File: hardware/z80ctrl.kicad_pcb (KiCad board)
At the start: 2 copper layers, 99.8 x 49.9 mm, 28 parts, among them J1 BUS, J2 BUSEXT, J4 IOADDR, J5 SERIAL1, J6 SERIAL2, J7 SD, SW1 RESET, SW2 HALT, U1 74HCT139, U2 ATMEGA1284P-PU, U3 74HCT74, U4 MCP23S17, Y1 20MHz

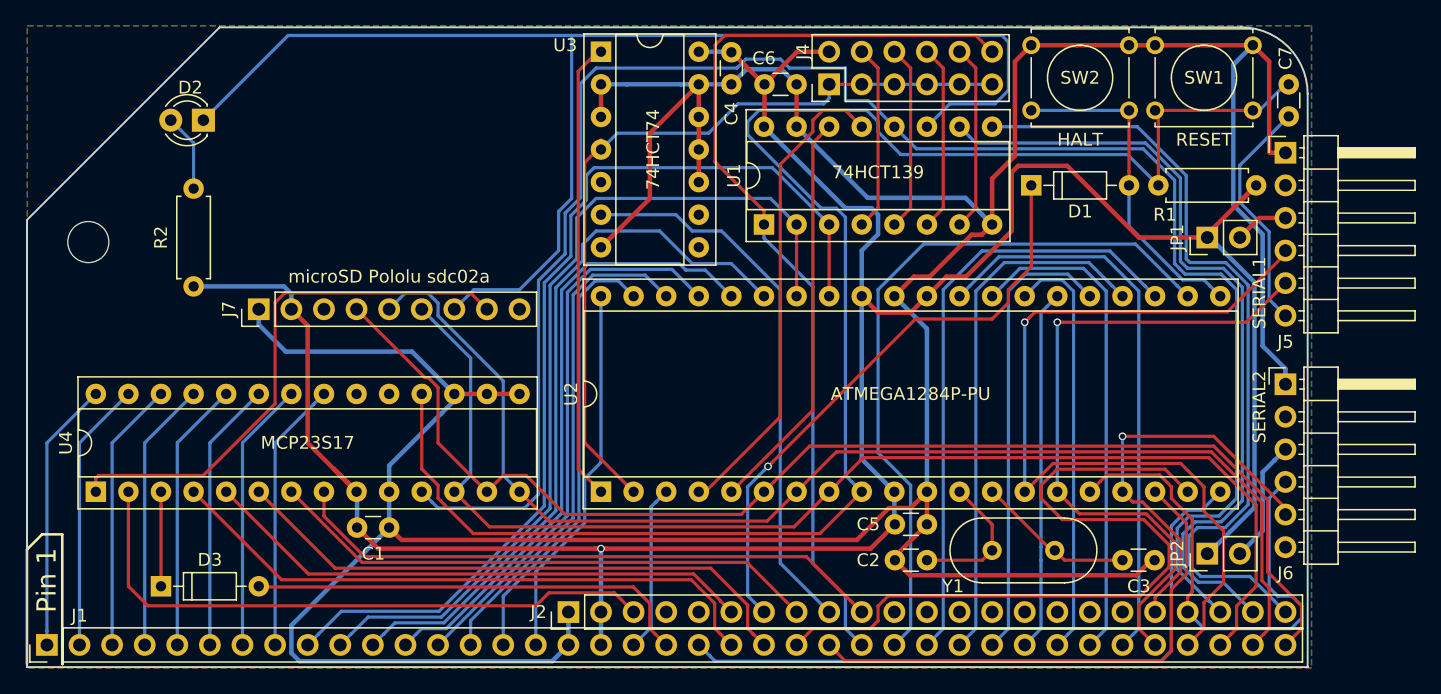
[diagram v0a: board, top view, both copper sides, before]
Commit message: OCD tweaks
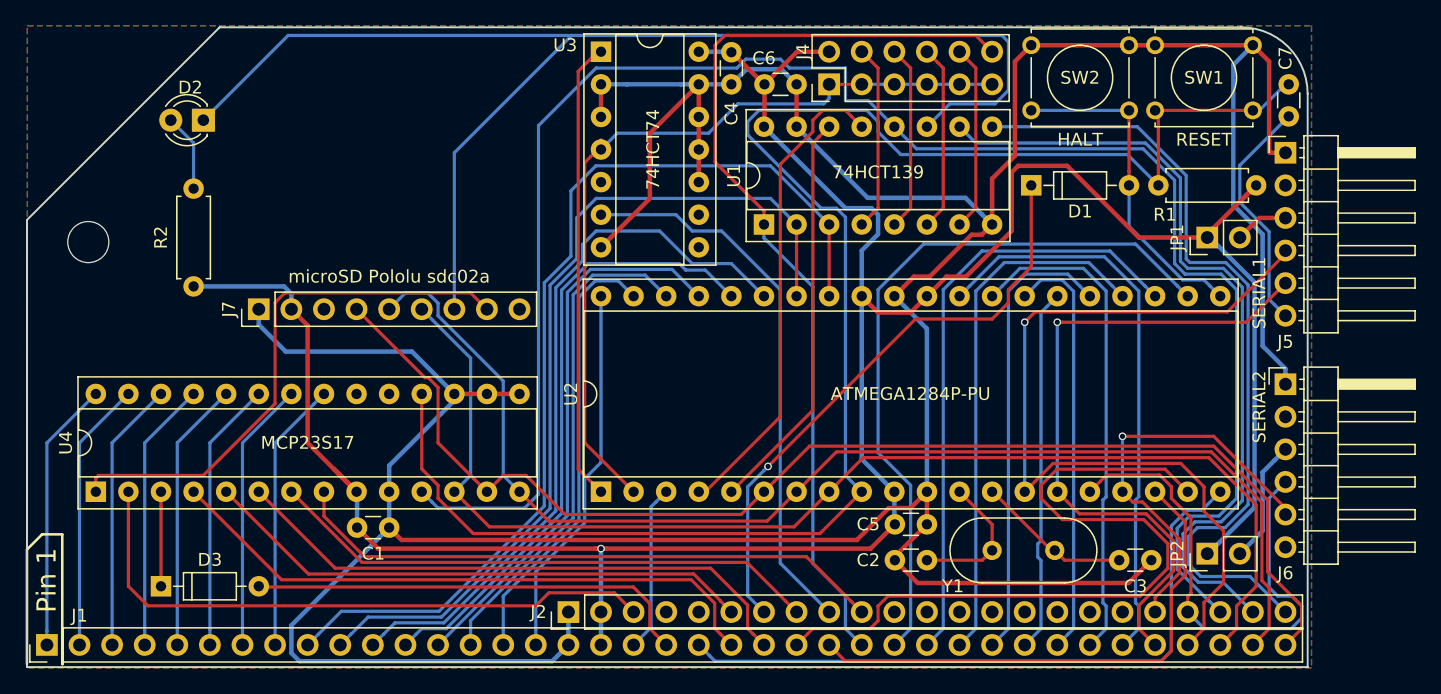
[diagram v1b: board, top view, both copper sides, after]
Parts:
- moved C3 0.25 mm to (239.3, 145.0)
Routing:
- net /SDCS: track 104.2 -> 102.1 mm
